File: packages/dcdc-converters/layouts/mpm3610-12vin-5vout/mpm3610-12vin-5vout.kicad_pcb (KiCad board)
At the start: 2 copper layers, 7 parts

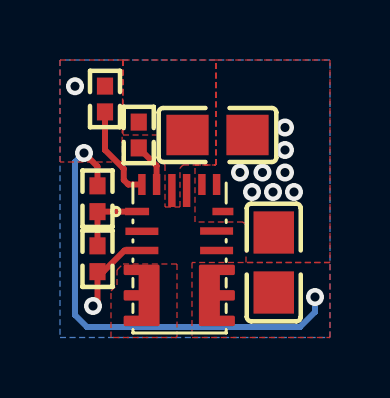
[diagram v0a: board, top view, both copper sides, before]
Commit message: WIP update dcdc converters
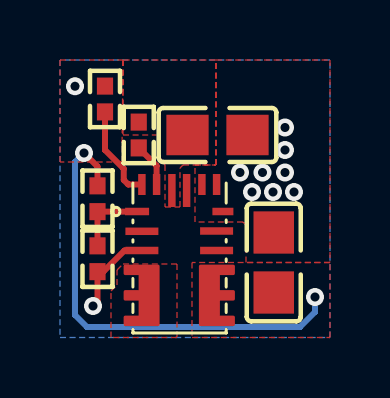
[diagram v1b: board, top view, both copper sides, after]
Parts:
- C1: footprint atopile:C0805-3b2e55 -> Samsung_Electro_Mechanics_CL21A106KAYNNNE:C0805
- C2: footprint atopile:C0805-3b2e55 -> Samsung_Electro_Mechanics_CL21A226KOQNNNE:C0805
- R1: footprint atopile:R0402-56259e -> UNI_ROYAL_0402WGF5362TCE:R0402
- R2, R4: footprint atopile:R0402-56259e -> YAGEO_RC0402FR_07100KL:R0402
- R3: footprint atopile:R0402-56259e -> UNI_ROYAL_0402WGF1912TCE:R0402
- U1: footprint atopile:QFN-20_L5.0-W3.0-TL-MPM3610GQV-Z-b63965 -> MONOLITHIC_POWER_SYSTEMS_INC_MPM3610GQV_Z:QFN-20_L5.0-W3.0-TL-MPM3610GQV-Z

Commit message: WIP update packages till ESPs
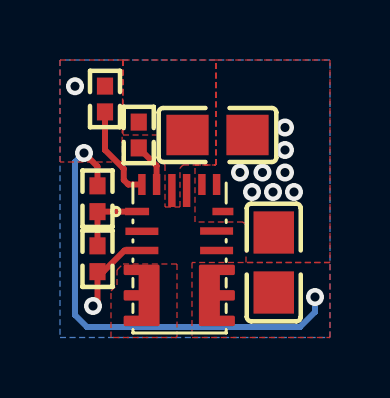
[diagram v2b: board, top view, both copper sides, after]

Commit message: Manually fix fp lib tables
fix some small bugs
fix package only modules (e.g. logos)
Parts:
- R2, R4: footprint YAGEO_RC0402FR_07100KL:R0402 -> UNI_ROYAL_0402WGF1003TCE:R0402

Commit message: Use packages from packages folder
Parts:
- C2: value 22µF ±10% 16V X5R -> 22µF ±10% 10V X5R; footprint Samsung_Electro_Mechanics_CL21A226KOQNNNE:C0805 -> CCTC_TCC0805X5R226K100FT:C0805
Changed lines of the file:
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@@
     (net 10 "IN")
     (net 11 "gnd")
-    (footprint "Samsung_Electro_Mechanics_CL21A226KOQNNNE:C0805"
+    (footprint "CCTC_TCC0805X5R226K100FT:C0805"
         (layer "F.Cu")
         (at 3.125 0.75 90)
@@
             )
         )
-        (property "Value" "22µF ±10% 16V X5R"
+        (property "Value" "22µF ±10% 10V X5R"
             (at 0 4 0)
             (layer "F.Fab")
@@
             )
         )
-        (property "Datasheet" "https://wmsc.lcsc.com/wmsc/upload/file/pdf/v2/lcsc/2304140030_Samsung-Electro-Mechanics-CL21A226KOQNNNE_C296720.pdf"
+        (property "Datasheet" "https://wmsc.lcsc.com/wmsc/upload/file/pdf/v2/lcsc/2304140030_CCTC-TCC0805X5R226K100FT_C380336.pdf"
             (at 0 0 0)
             (layer "F.Fab")
@@
             )
         )
-        (property "checksum" "48ef5b1f25a5a96ef742ee98536270bc2e83311e312c1247ec8696f866d4b5f5"
-            (at 0 0 0)
-            (layer "User.9")
-            (hide yes)
-            (effects
-                (font
-                    (size 0.125 0.125)
-                    (thickness 0.01875)
-                )
-            )
-        )
-        (property "__atopile_lib_fp_hash__" "13fc7ffd-ee7b-9770-b032-88b84d476fe6"
-            (at 0 0 0)
-            (layer "User.9")
-            (hide yes)
-            (effects
-                (font
-                    (size 0.125 0.125)
-                    (thickness 0.01875)
-                )
-            )
-        )
-        (property "LCSC" "C296720"
-            (at 0 0 90)
-            (layer "User.9")
-            (hide yes)
-            (effects
-                (font
-                    (size 0.125 0.125)
-                    (thickness 0.01875)
-                )
-            )
-        )
-        (property "Partnumber" "CL21A226KOQNNNE"
-            (at 0 0 90)
-            (layer "User.9")
-            (hide yes)
-            (effects
-                (font
-                    (size 0.125 0.125)
-                    (thickness 0.01875)
-                )
-            )
-        )
-        (property "Manufacturer" "Samsung Electro-Mechanics"
+        (property "checksum" "c92c130d59add2b9f30b35f755af606548a01fad9c9899b9e82df6ee5a8eead8"
+            (at 0 0 0)
+            (layer "User.9")
+            (hide no)
+            (effects
+                (font
+                    (size 0.125 0.125)
+                    (thickness 0.01875)
+                )
+                (hide yes)
+            )
+        )
+        (property "__atopile_lib_fp_hash__" "711beecb-e60a-bb27-b241-e86edd3e7434"
+            (at 0 0 0)
+            (layer "User.9")
+            (hide yes)
+            (effects
+                (font
+                    (size 0.125 0.125)
+                    (thickness 0.01875)
+                )
+            )
+        )
+        (property "LCSC" "C380336"
+            (at 0 0 90)
+            (layer "User.9")
+            (hide yes)
+            (effects
+                (font
+                    (size 0.125 0.125)
+                    (thickness 0.01875)
+                )
+            )
+        )
+        (property "Partnumber" "TCC0805X5R226K100FT"
+            (at 0 0 90)
+            (layer "User.9")
+            (hide yes)
+            (effects
+                (font
+                    (size 0.125 0.125)
+                    (thickness 0.01875)
+                )
+            )
+        )
+        (property "Manufacturer" "CCTC"
             (at 0 0 90)
             (layer "User.9")
@@
             )
         )
-        (property "PARAM_max_voltage" "{\"type\": \"Quantity_Set_Discrete\", \"data\": {\"intervals\": {\"type\": \"Numeric_Interval_Disjoint\", \"data\": {\"intervals\": [{\"type\": \"Numeric_Interval\", \"data\": {\"min\": 16.0, \"max\": 16.0}}]}}, \"unit\": \"volt\"}}"
+        (property "PARAM_max_voltage" "{\"type\": \"Quantity_Set_Discrete\", \"data\": {\"intervals\": {\"type\": \"Numeric_Interval_Disjoint\", \"data\": {\"intervals\": [{\"type\": \"Numeric_Interval\", \"data\": {\"min\": 10.0, \"max\": 10.0}}]}}, \"unit\": \"volt\"}}"
             (at 0 0 90)
             (layer "User.9")
@@
         )
         (fp_line
+            (start 0.4 0.9)
+            (end 1.81 0.9)
+            (stroke
+                (width 0.15)
+                (type solid)
+            )
+            (layer "F.SilkS")
+        )
+        (fp_line
+            (start 1.96 0.75)
+            (end 1.96 -0.75)
+            (stroke
+                (width 0.15)
+                (type solid)
+            )
+            (layer "F.SilkS")
+        )
+        (fp_line
             (start -1.81 -0.9)
             (end -0.4 -0.9)
@@
         )
         (fp_line
-            (start 1.96 0.75)
-            (end 1.96 -0.75)
+            (start -0.4 0.9)
+            (end -1.81 0.9)
             (stroke
                 (width 0.15)
@@
             (layer "F.SilkS")
         )
-        (fp_line
-            (start 0.4 0.9)
-            (end 1.81 0.9)
-            (stroke
-                (width 0.15)
-                (type solid)
-            )
-            (layer "F.SilkS")
-        )
-        (fp_line
-            (start -0.4 0.9)
-            (end -1.81 0.9)
+        (fp_arc
+            (start 1.96 0.75)
+            (mid 1.9160660171779822 0.856066017177982)
+            (end 1.81 0.8999999999999999)
             (stroke
                 (width 0.15)
@@
         (fp_arc
             (start 1.81 -0.9)
-            (mid 1.916066 -0.856066)
+            (mid 1.9160660171779822 -0.8560660171779821)
             (end 1.96 -0.75)
             (stroke
@@
         )
         (fp_arc
-            (start -1.96 -0.75)
-            (mid -1.916066 -0.856066)
-            (end -1.81 -0.9)
+            (start -1.96 0.75)
+            (mid -1.9160660171779822 0.856066017177982)
+            (end -1.81 0.8999999999999999)
             (stroke
                 (width 0.15)
@@
         )
         (fp_arc
-            (start 1.96 0.75)
-            (mid 1.916066 0.856066)
-            (end 1.81 0.9)
-            (stroke
-                (width 0.15)
-                (type solid)
-            )
-            (layer "F.SilkS")
-        )
-        (fp_arc
-            (start -1.81 0.9)
-            (mid -1.916066 0.856066)
-            (end -1.96 0.75)
+            (start -1.81 -0.9)
+            (mid -1.9160660171779822 -0.8560660171779821)
+            (end -1.96 -0.75)
             (stroke
                 (width 0.15)
@@
             (layer "F.Fab")
         )
+        (fp_text user "%R"
+            (at 0 0 0)
+            (layer "F.Fab")
+            (effects
+                (font
+                    (size 1 1)
+                    (thickness 0.15)
+                )
+            )
+            (unlocked no)
+        )
+        (fp_text user "${REFERENCE}"
+            (at 0 -4 0)
+            (layer "F.SilkS")
+            (effects
+                (font
+                    (size 1 1)
+                    (thickness 0.15)
+                )
+                (hide yes)
+            )
+            (unlocked no)
+        )
+        (pad "2" smd rect
+            (at 1 0 90)
+            (size 1.41 1.35)
+            (layers "F.Cu" "F.Paste" "F.Mask")
+            (net 11 "gnd")
+        )
         (pad "1" smd rect
             (at -1 0 90)
             (size 1.41 1.35)
-            (layers "F.Cu" "F.Mask" "F.Paste")
+            (layers "F.Cu" "F.Paste" "F.Mask")
             (net 1 "OUT")
         )
-        (pad "2" smd rect
-            (at 1 0 90)
-            (size 1.41 1.35)
-            (layers "F.Cu" "F.Mask" "F.Paste")
-            (net 11 "gnd")
-        )
-        (embedded_fonts no)
-        (model "${KIPRJMOD}/../../parts/Samsung_Electro_Mechanics_CL21A226KOQNNNE/C0805_L2.0-W1.3-H1.3.step"
+        (model "${KIPRJMOD}/../../parts/CCTC_TCC0805X5R226K100FT/C0805_L2.0-W1.3-H1.3.step"
             (offset
-                (xyz 0 0 0.6)
+                (xyz 0 0 0)
             )
             (scale
